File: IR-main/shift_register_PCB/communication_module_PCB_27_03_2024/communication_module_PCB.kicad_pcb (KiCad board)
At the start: 2 copper layers, 75 x 75 mm, 58 parts, among them U2 74LS08, U3 74LS08, U4 header-6

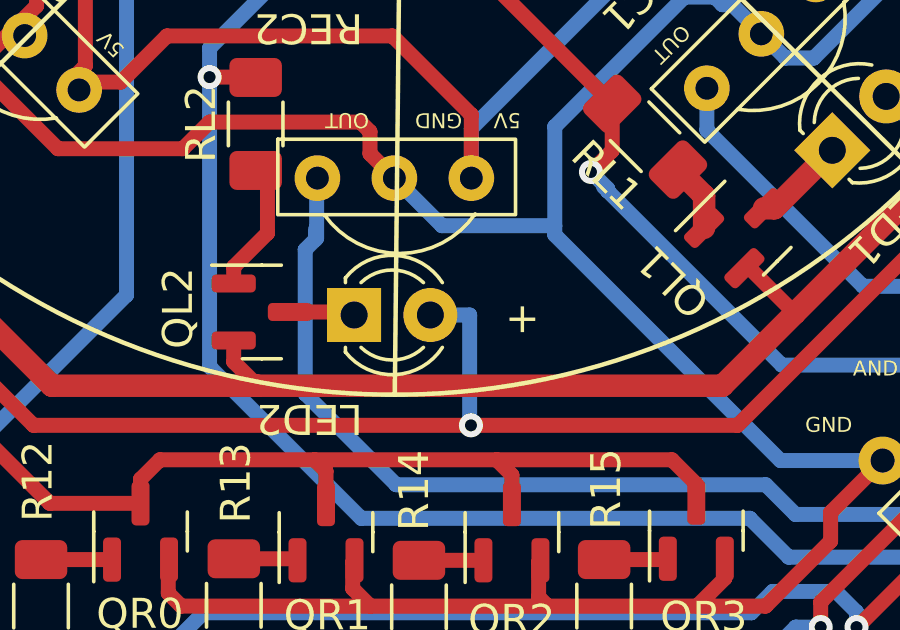
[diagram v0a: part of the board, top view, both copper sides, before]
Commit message: .
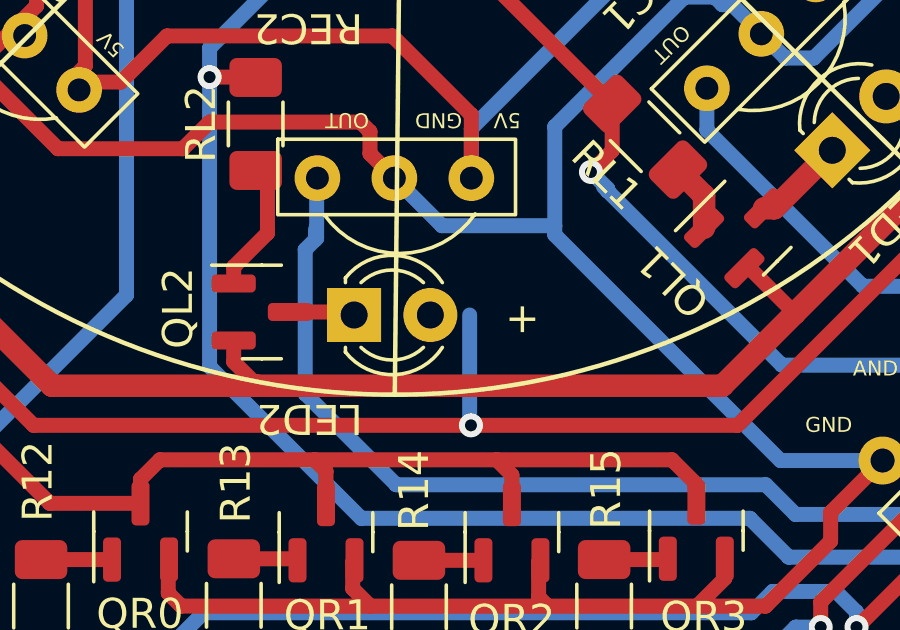
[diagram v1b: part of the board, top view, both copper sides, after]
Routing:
- net Net-(LED7-Pad2): track 187.1 -> 185.8 mm
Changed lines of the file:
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@@
   (via (at 64.9859 30.7467) (size 0.8) (drill 0.4) (layers "F.Cu" "B.Cu") (net 33))
   (via (at 66.9163 67.3227) (size 0.8) (drill 0.4) (layers "F.Cu" "B.Cu") (net 33))
-  (segment (start 50.059059 71.518971) (end 48.748 71.518971) (width 0.5) (layer "B.Cu") (net 33))
   (segment (start 22.008229 51.270771) (end 21.9583 51.3207) (width 0.5) (layer "B.Cu") (net 33))
   (segment (start 45.878059 24.186459) (end 45.8343 24.1427) (width 0.5) (layer "B.Cu") (net 33))

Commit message: .
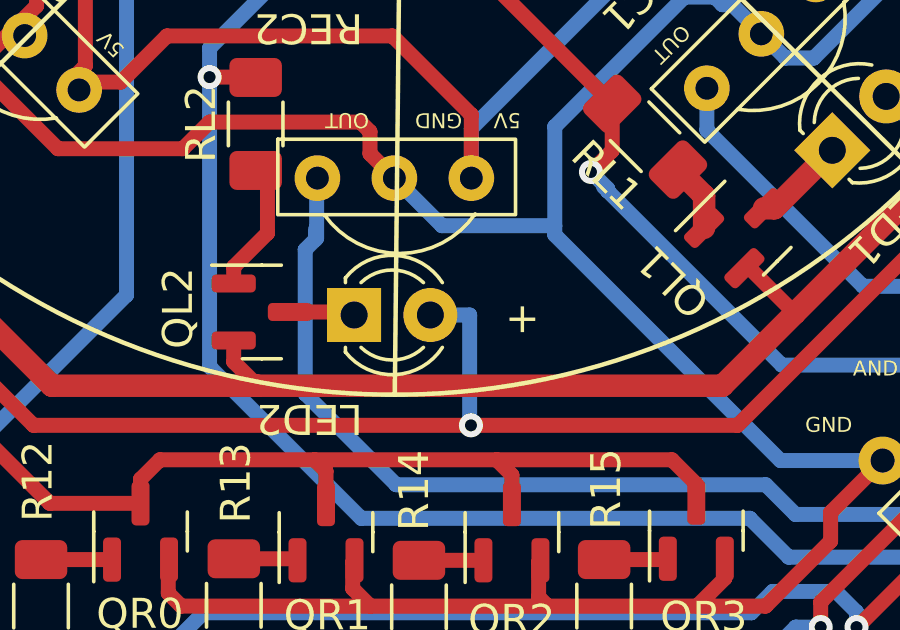
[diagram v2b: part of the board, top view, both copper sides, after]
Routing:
- net Net-(LED7-Pad2): track 185.8 -> 187.1 mm
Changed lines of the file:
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@@
   (via (at 64.9859 30.7467) (size 0.8) (drill 0.4) (layers "F.Cu" "B.Cu") (net 33))
   (via (at 66.9163 67.3227) (size 0.8) (drill 0.4) (layers "F.Cu" "B.Cu") (net 33))
+  (segment (start 50.059059 71.518971) (end 48.748 71.518971) (width 0.5) (layer "B.Cu") (net 33))
   (segment (start 22.008229 51.270771) (end 21.9583 51.3207) (width 0.5) (layer "B.Cu") (net 33))
   (segment (start 45.878059 24.186459) (end 45.8343 24.1427) (width 0.5) (layer "B.Cu") (net 33))
